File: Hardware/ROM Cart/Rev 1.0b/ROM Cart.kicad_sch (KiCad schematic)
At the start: 5 parts, among them J1 6502 Card Edge, U1 AT28C256, U2 74HC138

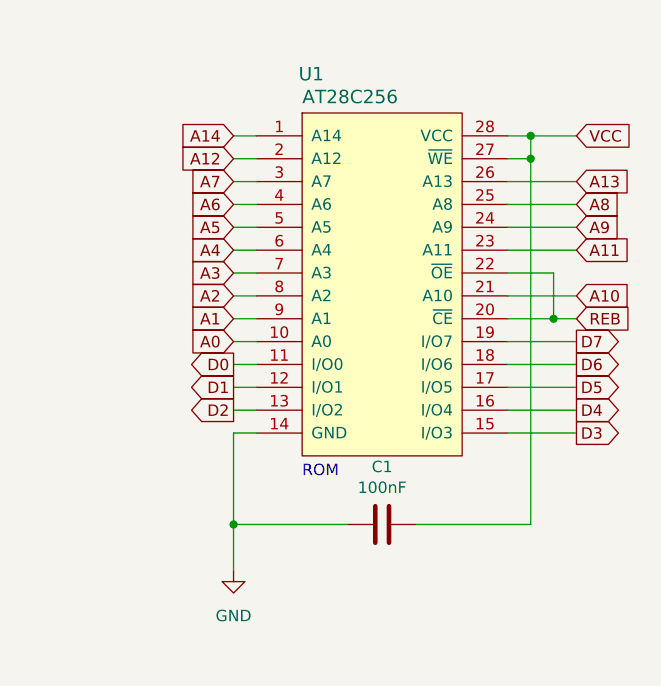
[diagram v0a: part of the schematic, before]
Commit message: Re-version ROM carts
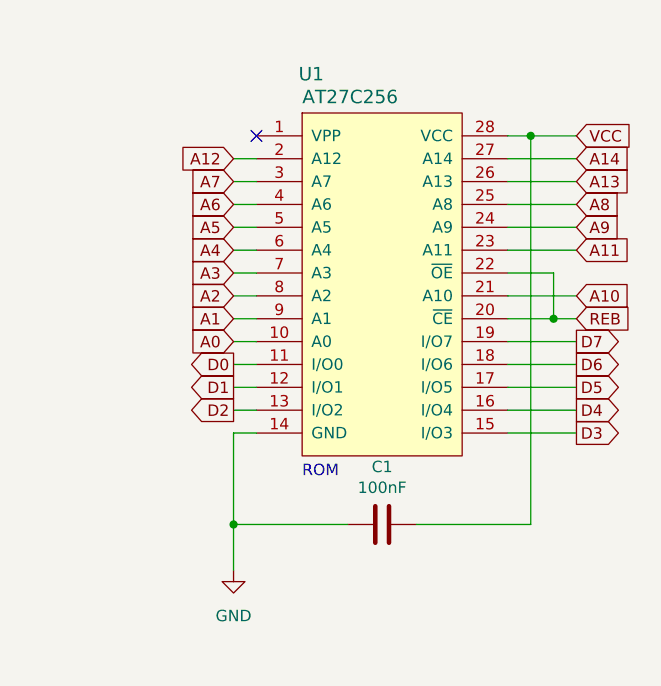
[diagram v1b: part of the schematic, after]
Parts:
- U1: value AT28C256 -> AT27C256; symbol 6502 Parts:AT28C256 -> 6502 Parts:AT27C256; now in the parts list
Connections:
- net A14: now also U1.27 (A14); no longer U1.1 (A14)
- net VCC: no longer U1.27 (~{WE})
- no-connect marks 15 -> 16
